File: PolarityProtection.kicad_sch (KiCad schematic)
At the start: 7 parts, among them Q201 BSC010N04LS, Q202 BSC010N04LS, U201 LM74502-Q1

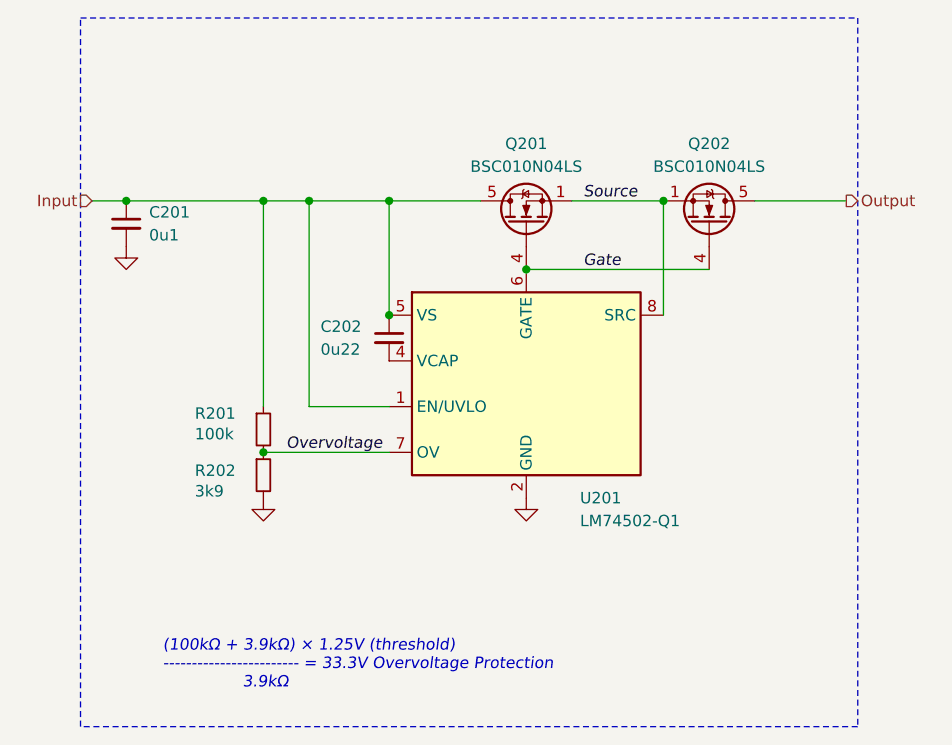
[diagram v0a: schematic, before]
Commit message: Update parts
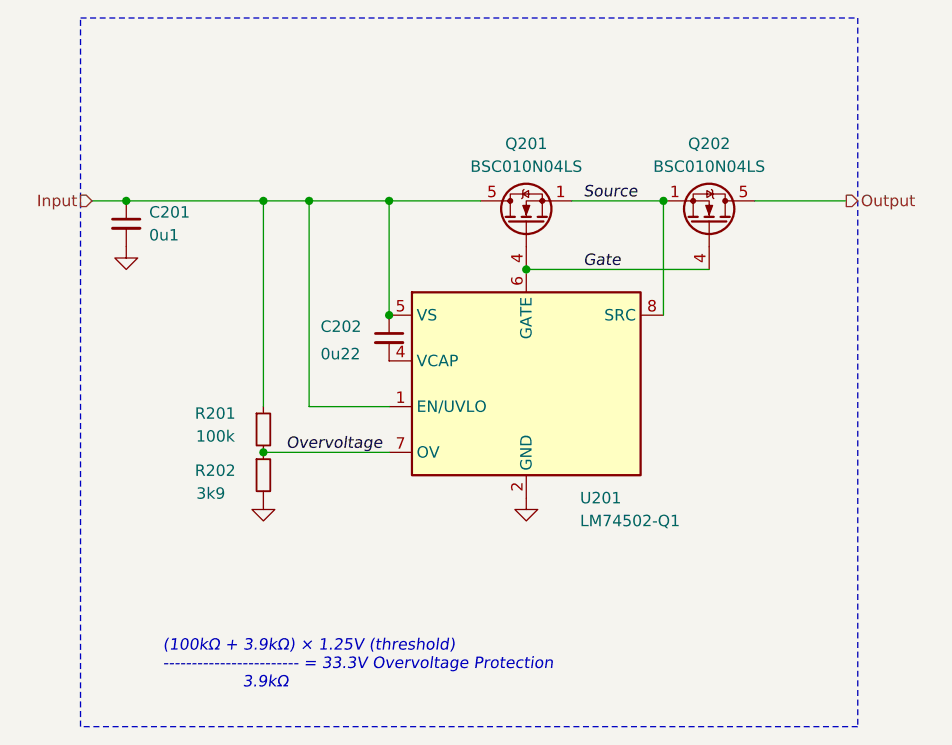
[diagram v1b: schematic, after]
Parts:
- C201: footprint Capacitor_SMD:C_0603_1608Metric -> V2_Capacitor_SMD:C_0603; symbol Device:C_Small -> V2_Device:C_0603_0u1; Manufacturer (none) -> TDK; Mouser (none) -> 810-CGA3E2X7R1H104MA; Product (none) -> CGA3E2X7R1H104M080AA
- C202: footprint Capacitor_SMD:C_0603_1608Metric -> V2_Capacitor_SMD:C_0603; symbol Device:C_Small -> V2_Device:C_0603_0u22; Manufacturer (none) -> YAGEO; Mouser (none) -> 603-CC0603JRX79BB224; Product (none) -> CC0603JRX7R9BB224
- Q201, Q202: Manufacturer (none) -> Infineon Technologies; Mouser (none) -> 726-BSC010N04LS; Product (none) -> BSC010N04LS
- R201: footprint Resistor_SMD:R_0603_1608Metric -> V2_Resistor_SMD:R_0603; symbol Device:R_Small -> V2_Device:R_0603_100k; Manufacturer (none) -> Vishay; Mouser (none) -> 71-CRCW0603100KFKEAC; Product (none) -> CRCW0603100KFKEAC; Rating (none) -> 100mW
- R202: footprint Resistor_SMD:R_0603_1608Metric -> V2_Resistor_SMD:R_0603; symbol Device:R_Small -> V2_Device:R_0603_3k9; Manufacturer (none) -> Vishay; Mouser (none) -> 71-CRCW06033K90FKEAC; Product (none) -> CRCW06033K90FKEAC; Rating (none) -> 100mW
- U201: Manufacturer (none) -> Texas Instruments; Mouser (none) -> 595-LM74502HQDDFRQ1; Product (none) -> LM74502HQDDFRQ1

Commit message: Update library
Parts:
- C201: Rating (none) -> 50V
- Q201, Q202: Polarity (none) -> N; Rating (none) -> 40V
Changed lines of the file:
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@@
-			)
-		)
-		(property "Sim.Pin" ""
-			(at 151.13 88.9 90)
-			(effects
-				(font
-					(size 1.27 1.27)
-				)
-				(hide yes)
 			)
 		)
@@
 		)
 		(property "Manufacturer" "Infineon Technologies"
+			(at 168.91 88.9 0)
+			(effects
+				(font
+					(size 1.27 1.27)
+				)
+				(hide yes)
+			)
+		)
+		(property "Rating" "40V"
+			(at 171.45 88.9 0)
+			(effects
+				(font
+					(size 1.27 1.27)
+				)
+				(hide yes)
+			)
+		)
+		(property "Polarity" "N"
 			(at 168.91 88.9 0)
 			(effects
@@
 			)
 		)
-		(property "Sim.Pin" ""
-			(at 151.13 106.68 0)
-			(effects
-				(font
-					(size 1.27 1.27)
-				)
-				(hide yes)
-			)
-		)
 		(property "Product" "LM74502HQDDFRQ1"
 			(at 151.13 144.78 0)
@@
 			)
 		)
-		(property "Sim.Pin" ""
-			(at 121.92 111.76 0)
-			(effects
-				(font
-					(size 1.27 1.27)
-				)
-				(hide yes)
-			)
-		)
 		(property "Rating" "100mW"
 			(at 121.92 132.08 0)
@@
 			)
 		)
-		(property "Description" "Power symbol creates a global label with name \"GND\" , ground"
+		(property "Description" ""
 			(at 106.68 91.44 0)
 			(effects
@@
 			)
 		)
-		(property "Sim.Pin" ""
-			(at 171.45 88.9 90)
-			(effects
-				(font
-					(size 1.27 1.27)
-				)
-				(hide yes)
-			)
-		)
 		(property "Product" "BSC010N04LS"
 			(at 151.13 88.9 0)
@@
 		)
 		(property "Manufacturer" "Infineon Technologies"
+			(at 153.67 88.9 0)
+			(effects
+				(font
+					(size 1.27 1.27)
+				)
+				(hide yes)
+			)
+		)
+		(property "Rating" "40V"
+			(at 151.13 88.9 0)
+			(effects
+				(font
+					(size 1.27 1.27)
+				)
+				(hide yes)
+			)
+		)
+		(property "Polarity" "N"
 			(at 153.67 88.9 0)
 			(effects
@@
 			)
 		)
-		(property "Sim.Pin" ""
-			(at 106.68 88.9 0)
-			(effects
-				(font
-					(size 1.27 1.27)
-				)
-				(hide yes)
-			)
-		)
 		(property "Manufacturer" "TDK"
 			(at 106.68 104.14 0)
@@
 		(property "Product" "CGA3E2X7R1H104M080AA"
 			(at 106.68 106.68 0)
+			(effects
+				(font
+					(size 1.27 1.27)
+				)
+				(hide yes)
+			)
+		)
+		(property "Rating" "50V"
+			(at 106.68 111.76 0)
 			(effects
 				(font
@@
 			)
 		)
-		(property "Sim.Pin" ""
-			(at 135.89 101.6 0)
-			(effects
-				(font
-					(size 1.27 1.27)
-				)
-				(hide yes)
-			)
-		)
 		(property "Product" "CC0603JRX7R9BB224"
 			(at 135.89 119.38 0)
@@
 			)
 		)
-		(property "Sim.Pin" ""
-			(at 121.92 116.84 0)
-			(effects
-				(font
-					(size 1.27 1.27)
-				)
-				(hide yes)
-			)
-		)
 		(property "Product" "CRCW06033K90FKEAC"
 			(at 121.92 134.62 0)
@@
 			)
 		)
-		(property "Description" "Power symbol creates a global label with name \"GND\" , ground"
+		(property "Description" ""
 			(at 151.13 119.38 0)
 			(effects
@@
 			)
 		)
-		(property "Description" "Power symbol creates a global label with name \"GND\" , ground"
+		(property "Description" ""
 			(at 121.92 119.38 0)
 			(effects

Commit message: Use date as revision
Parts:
- U201: Mouser 595-LM74502HQDDFRQ1 -> 595-LM74502QDDFRQ1; Product LM74502HQDDFRQ1 -> LM74502QDDFRQ1
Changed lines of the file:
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@@
 			)
 		)
-		(property "Mouser" "595-LM74502HQDDFRQ1"
+		(property "Mouser" "595-LM74502QDDFRQ1"
 			(at 151.13 106.68 0)
 			(effects
@@
 			)
 		)
-		(property "Product" "LM74502HQDDFRQ1"
+		(property "Product" "LM74502QDDFRQ1"
 			(at 151.13 144.78 0)
 			(effects

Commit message: Update Library
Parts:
- C201: symbol V2_Device:C_0603_0u1 -> V2_Capacitor:0603_0u1
- C202: symbol V2_Device:C_0603_0u22 -> V2_Capacitor:0603_0u22
- R201: symbol V2_Device:R_0603_100k -> V2_Resistor:0603_100k
- R202: symbol V2_Device:R_0603_3k9 -> V2_Resistor:0603_3k9
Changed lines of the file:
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@@
 	)
 	(symbol
-		(lib_id "V2_Device:R_0603_100k")
+		(lib_id "V2_Resistor:0603_100k")
 		(at 121.92 111.76 0)
 		(unit 1)
@@
 	)
 	(symbol
-		(lib_id "V2_Device:C_0603_0u1")
+		(lib_id "V2_Capacitor:0603_0u1")
 		(at 106.68 88.9 0)
 		(unit 1)
@@
 	)
 	(symbol
-		(lib_id "V2_Device:C_0603_0u22")
+		(lib_id "V2_Capacitor:0603_0u22")
 		(at 135.89 101.6 0)
 		(unit 1)
@@
 	)
 	(symbol
-		(lib_id "V2_Device:R_0603_3k9")
+		(lib_id "V2_Resistor:0603_3k9")
 		(at 121.92 116.84 0)
 		(unit 1)
